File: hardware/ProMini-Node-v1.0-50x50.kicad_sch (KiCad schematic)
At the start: 17 parts, among them P1 Ant_SMA, P2 Power Input, P3 CONN_1, P4 CONN_2, P5 CONN_3, P6 CONN_4, P7 Ant, P8 Ant_uFL, P9 CONN_4, Q1 BSS84, U1 RFM95HW

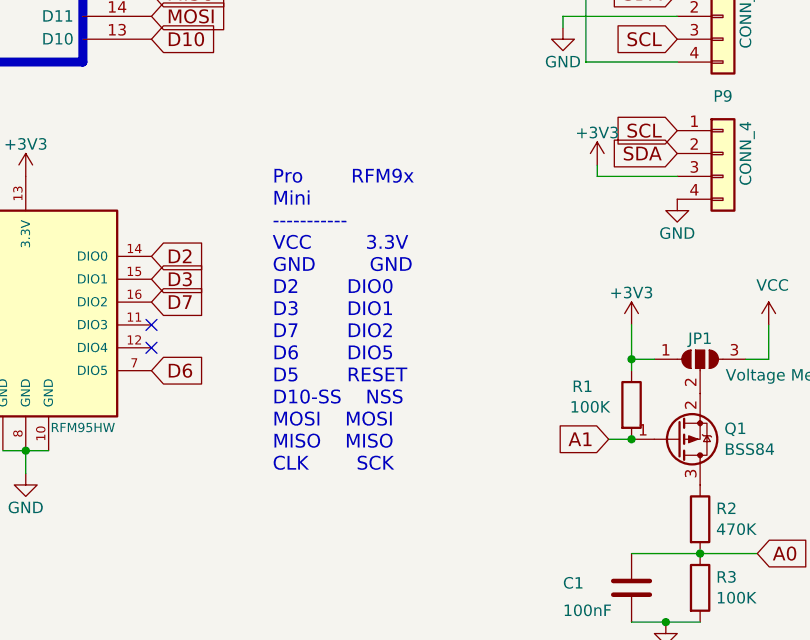
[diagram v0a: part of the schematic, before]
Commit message: example firmware update
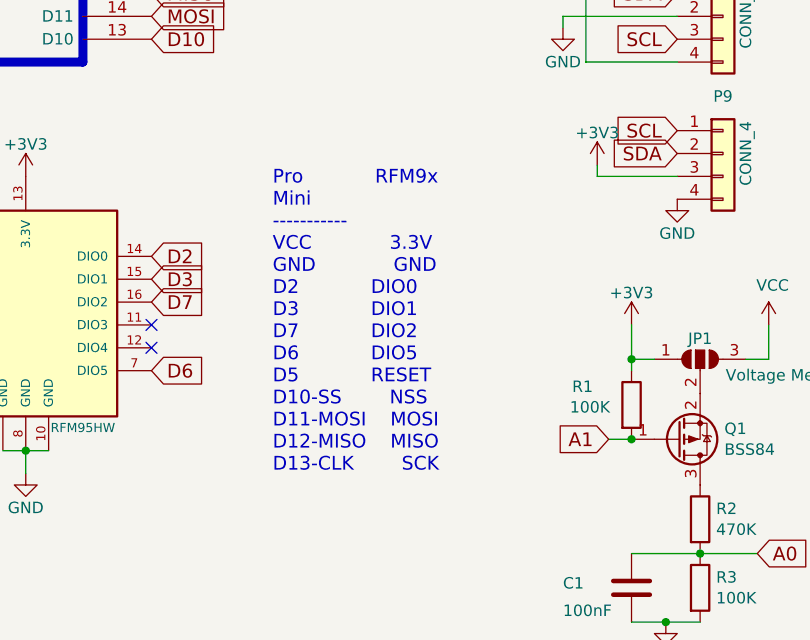
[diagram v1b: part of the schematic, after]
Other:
- note added: "Pro RFM9x Mini ----------- VCC 3.3V GND GND D2 DIO0 D3 DIO1 D7 DIO2 D6 DIO5 D5 RESET D10-SS NSS D11-MOSI MOSI D12-MISO MISO D13-CLK SCK"
- note removed: "Pro RFM9x Mini ----------- VCC 3.3V GND GND D2 DIO0 D3 DIO1 D7 DIO2 D6 DIO5 D5 RESET D10-SS NSS MOSI MOSI MISO MISO CLK SCK"
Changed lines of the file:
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@@
 		)
 	)
-	(text "Pro		RFM9x	\nMini\n-----------\nVCC	 	3.3V\nGND	 	GND	 \nD2		DIO0	 \nD3		DIO1\nD7		DIO2	 \nD6		DIO5\nD5		RESET	 	 \nD10-SS	NSS	 \nMOSI	MOSI	 \nMISO	MISO	 \nCLK		SCK"
+	(text "Pro			RFM9x	\nMini\n-----------\nVCC	 		3.3V\nGND	 		GND	 \nD2			DIO0	 \nD3			DIO1\nD7			DIO2	 \nD6			DIO5\nD5			RESET	 	 \nD10-SS		NSS	 \nD11-MOSI	MOSI	 \nD12-MISO	MISO	 \nD13-CLK		SCK"
 		(exclude_from_sim no)
 		(at 179.832 138.43 0)
